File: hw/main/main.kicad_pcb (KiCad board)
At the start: 2 copper layers, 91.3 x 100 mm, 44 parts, among them J1 Control A, J2 Control Pwr, J3 LCD, J4 Power, J5 Control D, J6 DAC Out, U1 MCP4821, U2 MCP3208, U3 LM4040C30, U4 LM4040C30, U5 TL072, U6 LMR50410

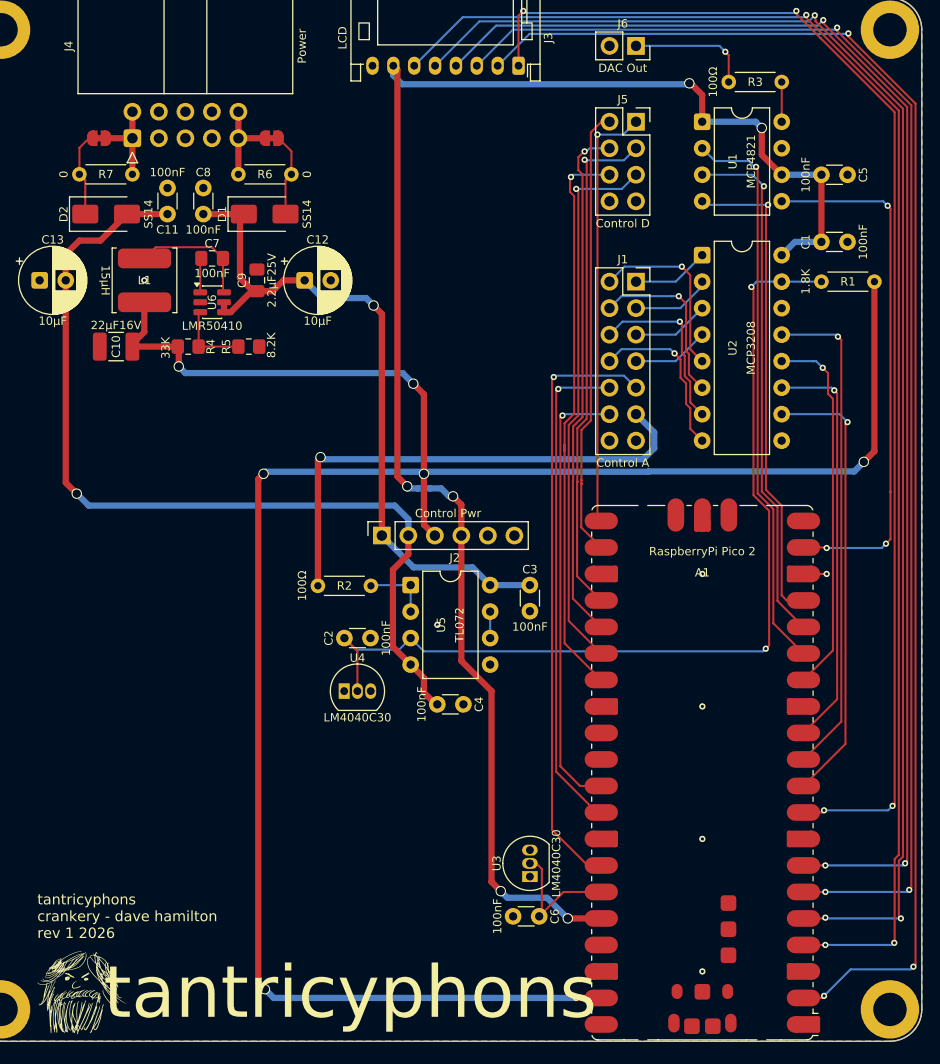
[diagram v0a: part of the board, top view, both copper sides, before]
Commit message: ordered rev 1
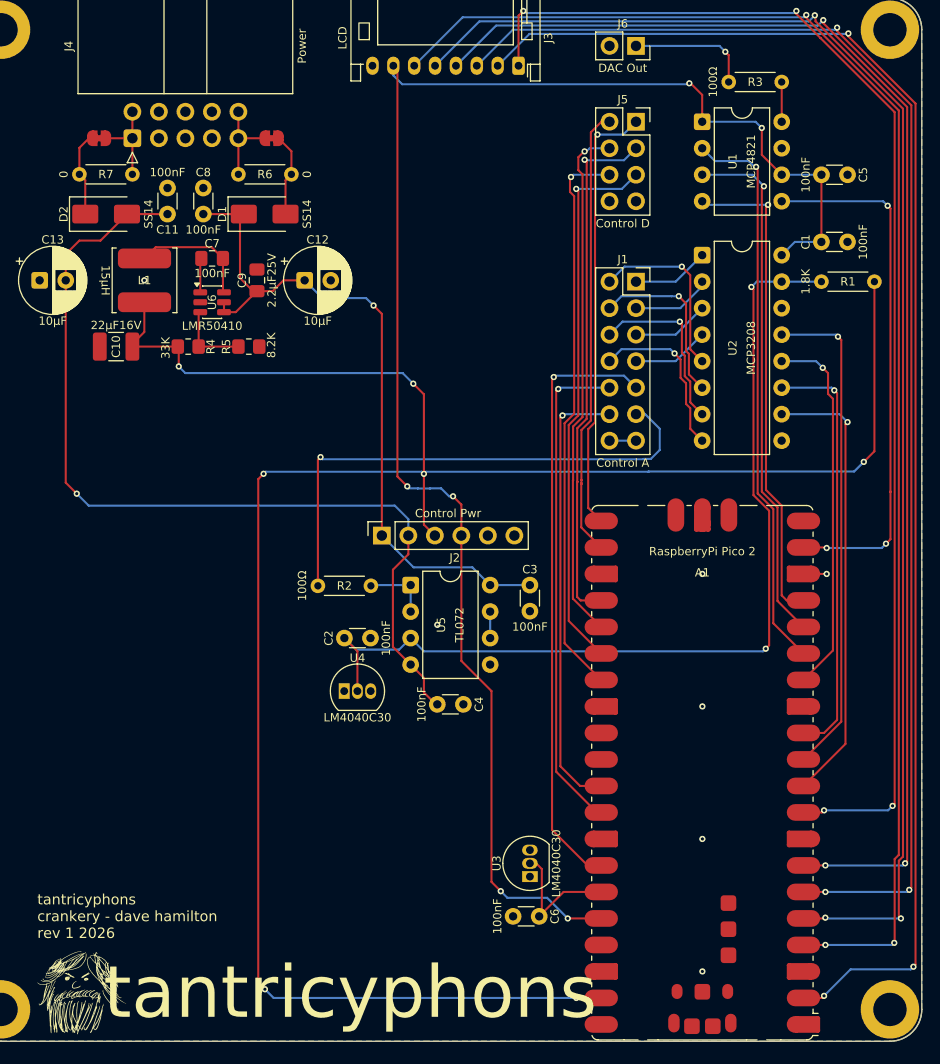
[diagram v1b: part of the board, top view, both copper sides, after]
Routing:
- net GND: track 2.23 -> 4.77 mm
- net /VREF_3V0_BUF: track 48.9 -> 50.3 mm
- net /ADC_DIN: track 39.4 -> 40.6 mm
- net /ENCODER_SW: track 49.1 -> 50.2 mm
- net +12V: track 68.6 -> 67.5 mm
- net /ENCODER_A: track 40.9 -> 41.6 mm
- net /MIDI_RX: track 54.7 -> 54.0 mm
- net +3.3V: track 156.0 -> 155.4 mm
